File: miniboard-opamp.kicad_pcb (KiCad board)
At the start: 2 copper layers, 22 parts, among them P1 CONN_01X03, P3 CONN_01X03, P4 CONN_01X03, U1 L78L12, U2 L79L12, U3 TL072

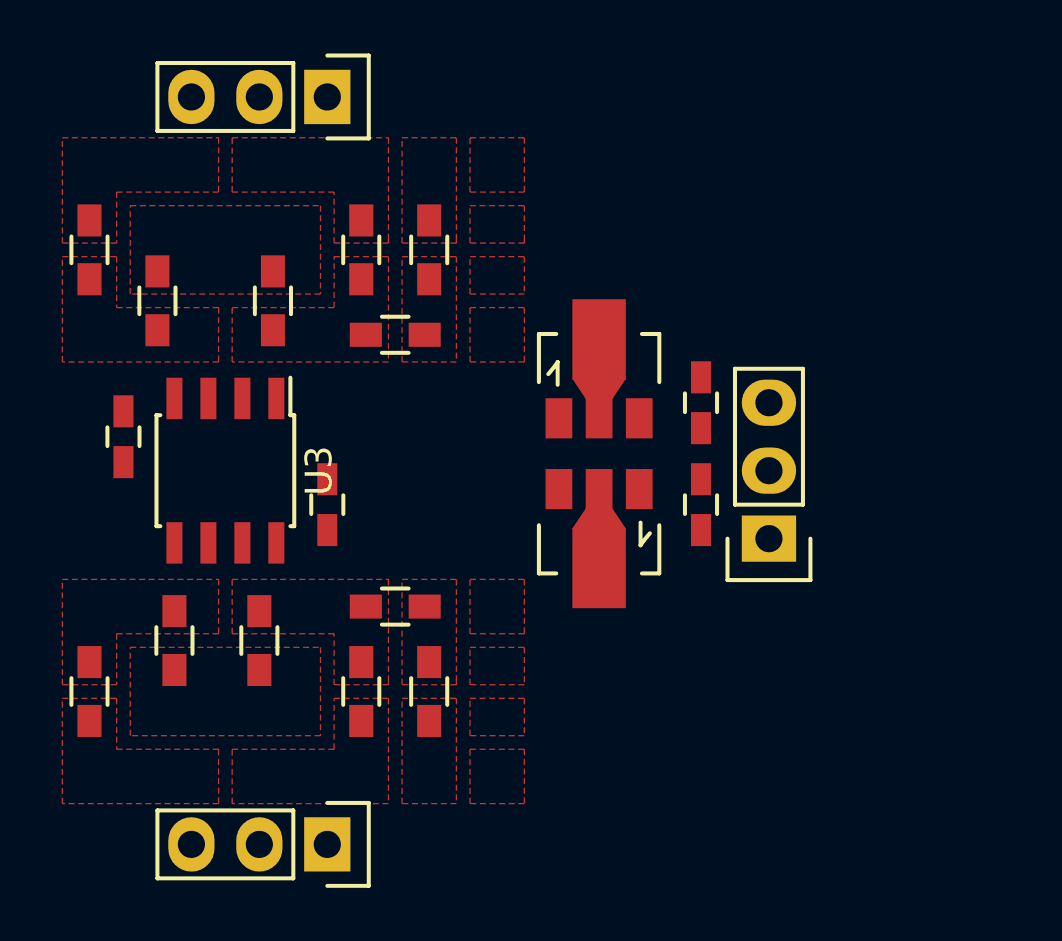
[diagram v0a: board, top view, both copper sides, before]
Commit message: 1st version finished
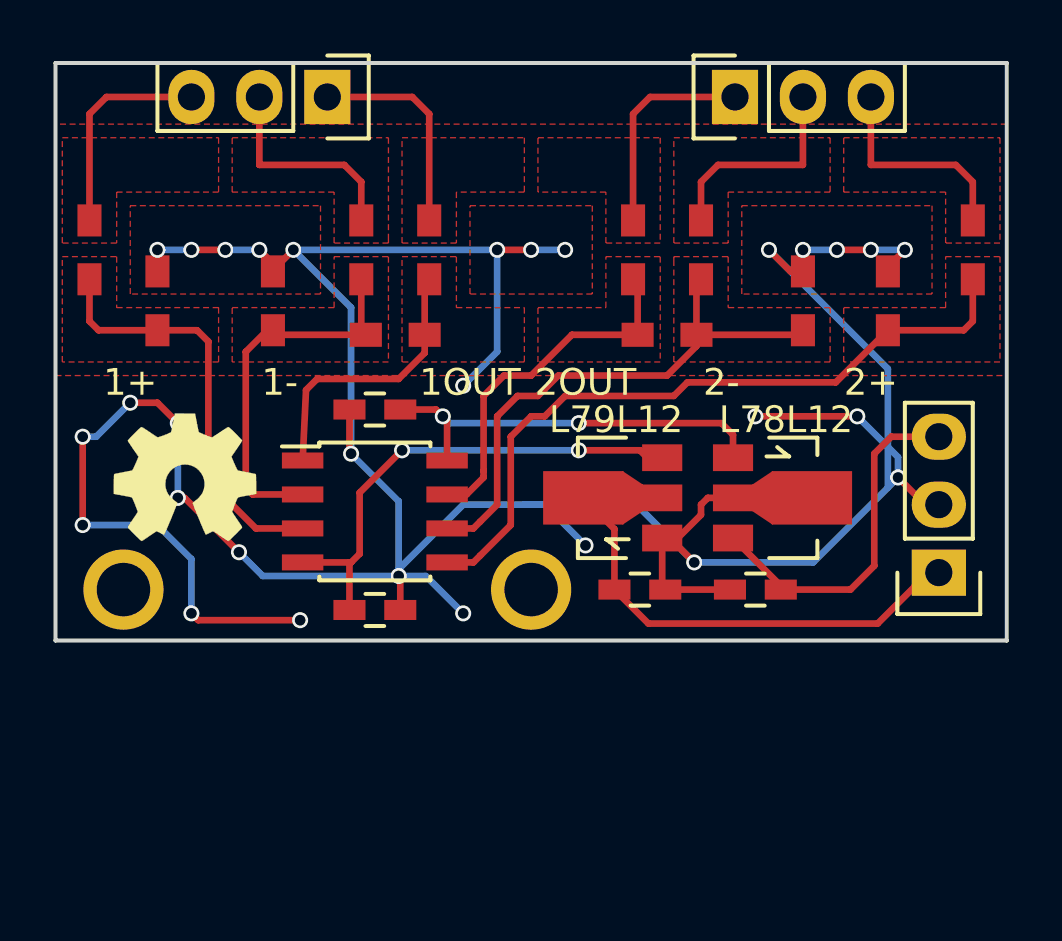
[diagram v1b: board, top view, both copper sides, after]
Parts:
- added G***: LOGO, oshw:logo_xs, F.Cu at (162.3, 93.0)
- added hole_2mm: VAL**, mechanics:hole_2mm, F.Cu at (160.0, 97.2)
- added hole_2mm: VAL**, mechanics:hole_2mm, F.Cu at (175.3, 97.2)
- added hole_2mm: VAL**, mechanics:hole_2mm, F.Cu at (196.2, 76.2)
- R1, R10, R11, R12, R2, R3, R4, R5, R6, R7, R8, R9: footprint Resistors_SMD:R_0603_HandSoldering -> pad:R_0603_nodraw
- moved R6 36.9 mm to (191.8, 84.5), turned to 90 degrees
- moved P4 31.8 mm to (182.9, 78.7), turned to 0 degrees
- moved R8 29.5 mm to (188.6, 86.4), turned to 90 degrees
- moved R9 24.0 mm to (185.4, 86.4), turned to 270 degrees
- moved R7 20.8 mm to (181.6, 84.5), turned to 90 degrees
- moved R12 18.2 mm to (179.1, 84.5), turned to 90 degrees
- moved R10 14.4 mm to (180.3, 87.6), turned to 0 degrees
- moved C4 11.4 mm to (169.4, 97.9), turned to 180 degrees
- moved U1 8.39 mm to (184.7, 93.7), turned to 270 degrees
- moved C1 7.27 mm to (183.6, 97.2), turned to 180 degrees
- moved P1 6.48 mm to (190.5, 96.5)
- moved U3 5.79 mm to (169.4, 94.2), turned to 0 degrees
- moved C3 3.98 mm to (169.4, 90.4), turned to 180 degrees
- moved C2 3.91 mm to (179.3, 97.2), turned to 180 degrees
- moved U2 1.61 mm to (178.3, 93.7), turned to 90 degrees
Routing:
- net GND: track 0.00 -> 137.6 mm, vias 0 -> 30
- net Net-(R6-Pad1): track 0.00 -> 26.9 mm
- net Net-(C2-Pad2): track 0.00 -> 21.4 mm
- net Net-(R10-Pad2): track 0.00 -> 21.3 mm
- net /-12_filter: track 0.00 -> 18.5 mm, vias 0 -> 2
- net Net-(R1-Pad1): track 0.00 -> 15.8 mm
- net /12_filter: track 0.00 -> 15.4 mm, vias 0 -> 2
- net Net-(R2-Pad1): track 0.00 -> 14.3 mm
- net Net-(R10-Pad1): track 0.00 -> 14.1 mm
- net Net-(C1-Pad1): track 0.00 -> 13.4 mm
- net Net-(R11-Pad1): track 0.00 -> 10.6 mm
- net Net-(P3-Pad3): track 0.00 -> 8.05 mm
- net Net-(P3-Pad2): track 0.00 -> 8.05 mm
- net Net-(P3-Pad1): track 0.00 -> 8.05 mm
- net Net-(P4-Pad3): track 0.00 -> 8.05 mm
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- added copper zone on B.Cu, net GND
- removed copper zone on F.Cu, net (none)
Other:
- board outline added: 35.6 x 21.6 mm
- board text added: "1+"
- board text added: "1-"
- board text added: "1OUT"
- board text added: "2+"
- board text added: "2-"
- board text added: "2OUT"
